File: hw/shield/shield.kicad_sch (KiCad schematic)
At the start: 6 parts, among them J2 DE9, Q1 PMOS, U1 TCAN330G, U2 MAX485E, U3 TPS5405DR

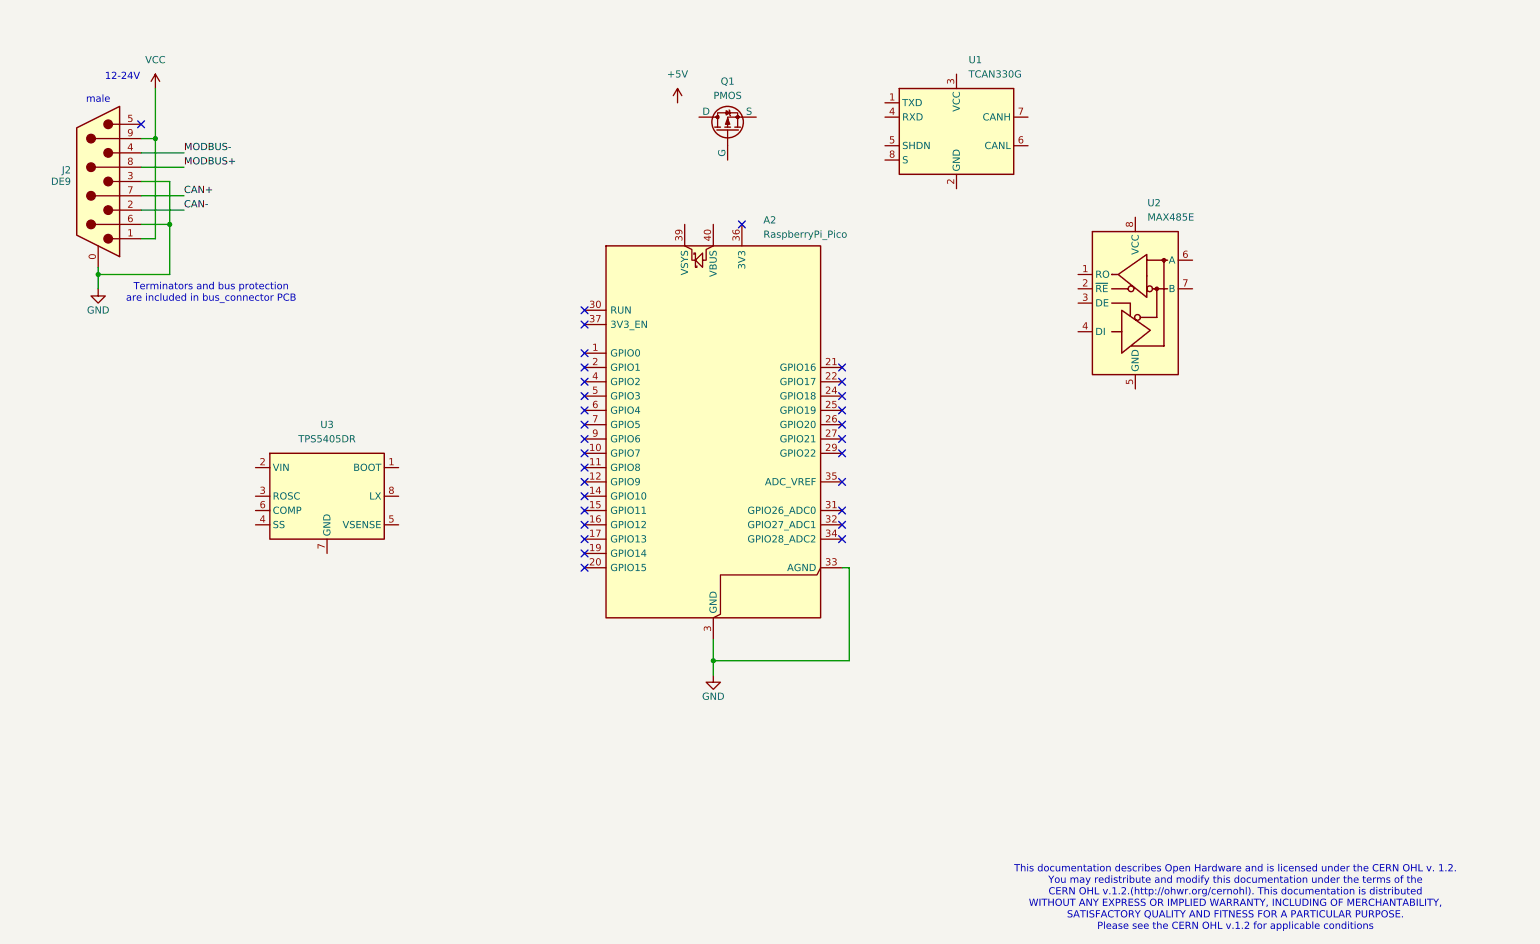
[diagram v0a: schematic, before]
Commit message: WIP shield
Signed-off-by: Mateusz Pająk <22417805+Tai-Min@users.noreply.github.com>
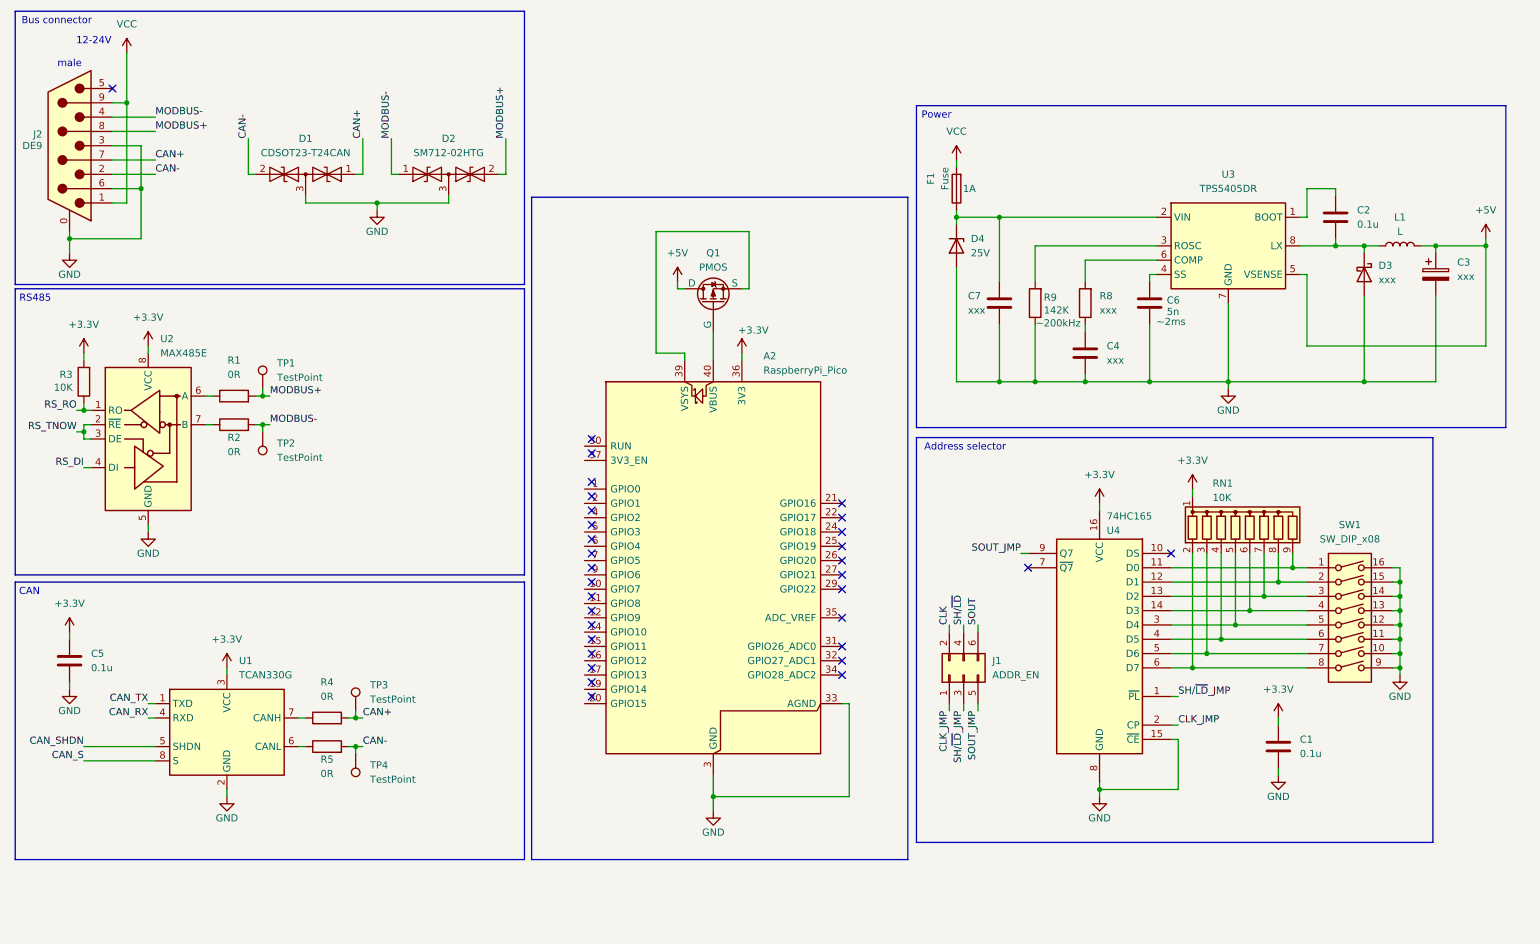
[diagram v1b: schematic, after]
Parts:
- added C1, C2, C5: 0.1u, symbol Device:C
- added C3: xxx, symbol Device:C_Polarized
- added C4, C7: xxx, symbol Device:C
- added C6: 5n, symbol Device:C
- added D1: CDSOT23-T24CAN, Package_TO_SOT_SMD:SOT-23, symbol Diode:SM712_SOT23
- added D2: SM712-02HTG, Package_TO_SOT_SMD:SOT-23, symbol Diode:SM712_SOT23
- added D3: xxx, symbol Device:D_Schottky
- added D4: 25V, symbol Device:D_Zener
- added F1: Fuse, symbol Device:Fuse
- added J1: ADDR_EN, symbol Connector_Generic:Conn_02x03_Odd_Even
- added L1: L, symbol Device:L
- added R1, R2, R4, R5: 0R, symbol Device:R
- added R3: 10K, symbol Device:R
- added R8: xxx, symbol Device:R
- added R9: 142K, symbol Device:R
- added RN1: 10K, Resistor_THT:R_Array_SIP9, symbol Device:R_Network08
- added SW1: SW_DIP_x08, Button_Switch_SMD:SW_DIP_SPSTx08_Slide_KingTek_DSHP08TS_W7.62mm_P1.27mm, symbol Switch:SW_DIP_x08
- added TP1, TP2, TP3, TP4: TestPoint, TestPoint:TestPoint_Pad_D1.5mm, symbol Connector:TestPoint
- added U4: 74HC165, Package_SO:SOIC-16_3.9x9.9mm_P1.27mm, symbol 74xx:74HC165
- U1: footprint (none) -> Package_SO:SOIC-8-1EP_3.9x4.9mm_P1.27mm_EP2.29x3mm
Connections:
- net +5V: now also Q1.1 (D), U3.5 (VSENSE), C3.1, L1.2
- net CAN+: now also D1.1 (A1), R4.2, TP3.1
- net CAN-: now also D1.2 (A2), R5.2, TP4.1
- net GND: now also U1.2 (GND), U2.5 (GND), U3.7 (GND), C1.2, C3.2, C4.1, C5.2, C6.1, C7.1, D1.3 (common), D2.3 (common), D3.2 (A), D4.2 (A), R9.1, SW1.10, SW1.11, SW1.12, SW1.13, SW1.14, SW1.15, SW1.16, SW1.9, U4.15 (~{CE}), U4.8 (GND)
- net MODBUS+: now also D2.2 (A2), R1.2, TP1.1
- net MODBUS-: now also D2.1 (A1), R2.2, TP2.1
- net VCC: now also F1.2
- net RS_RO: now reaches U2.1 (RO)
- net RS_RO: now also R3.1
- net RS_TNOW: now reaches U2.2 (~{RE})
- net RS_TNOW: now also U2.3 (DE)
- net RS_DI: now reaches U2.4 (DI)
- net at U2.6 (A): now also R1.1
- net at U2.7 (B): now also R2.1
- net +3.3V: now reaches U2.8 (VCC)
- net +3.3V: now also A2.36 (3V3), U1.3 (VCC), C1.1, C5.1, R3.2, RN1.1 (common), U4.16 (VCC)
- net at U3.1 (BOOT): now also C2.1
- net at U3.2 (VIN): now also C7.2, D4.1 (K), F1.1
- net at U3.3 (ROSC): now also R9.2
- net at U3.4 (SS): now also C6.2
- net at U3.6 (COMP): now also R8.2
- net at U3.8 (LX): now also C2.2, D3.1 (K), L1.1
- net CAN_TX: now reaches U1.1 (TXD)
- net CAN_RX: now reaches U1.4 (RXD)
- net CAN_SHDN: now reaches U1.5 (SHDN)
- net at U1.6 (CANL): now also R5.1
- net at U1.7 (CANH): now also R4.1
- net CAN_S: now reaches U1.8 (S)
- net at A2.39 (VSYS): now also Q1.3 (S)
- net at A2.40 (VBUS): now also Q1.2 (G)
- new net: C4.2, R8.1
- new net: RN1.9 (R8), SW1.1, U4.11 (D0)
- new net: RN1.8 (R7), SW1.2, U4.12 (D1)
- new net: RN1.7 (R6), SW1.3, U4.13 (D2)
- new net: RN1.6 (R5), SW1.4, U4.14 (D3)
- new net: RN1.5 (R4), SW1.5, U4.3 (D4)
- new net: RN1.4 (R3), SW1.6, U4.4 (D5)
- new net: RN1.3 (R2), SW1.7, U4.5 (D6)
- new net: RN1.2 (R1), SW1.8, U4.6 (D7)
- new net CLK: J1.2 (Pin_2)
- new net CLK_JMP: J1.1 (Pin_1), U4.2 (CP)
- new net SH/~{LD}: J1.4 (Pin_4)
- new net SH/~{LD}_JMP: J1.3 (Pin_3), U4.1 (~{PL})
- new net SOUT: J1.6 (Pin_6)
- new net SOUT_JMP: J1.5 (Pin_5), U4.9 (Q7)
- no-connect marks 31 -> 32
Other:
- note added: "Address selector"
- note added: "Bus connector"
- note added: "CAN"
- note added: "Power"
- note added: "RS485"
- note removed: "Terminators and bus protection are included in bus_connector PCB"
- note removed: "This documentation describes Open Hardware and is licensed under the CERN OHL v. 1.2. You may redistribute and modify this documentation under the terms of the CERN OHL v.1.2.(http://ohwr.org/cernohl). This documentation is distributed WITHOUT ANY EXPRESS OR IMPLIED WARRANTY, INCLUDING OF MERCHANTABILITY, SATISFACTORY QUALITY AND FITNESS FOR A PARTICULAR PURPOSE. Please see the CERN OHL v.1.2 for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"
- moved on the sheet: A2, J2, Q1, U1, U2, U3
